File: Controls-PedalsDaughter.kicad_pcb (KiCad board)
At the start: 2 copper layers, 49.2 x 70.5 mm, 54 parts, among them J1 Brake Pos. Sensor, J2 Accel Pos. Sensor, J3 PeripheralCANConnector, J4 Conn_01x02, J5 PeripheralCANConnector, U1 RI3-1205S, U2 PeripheralSOM, U3 TLV9301xDCK, U4 TLV70130DBVR, U5 AMC1300BDWV, U6 TLV9301xDCK

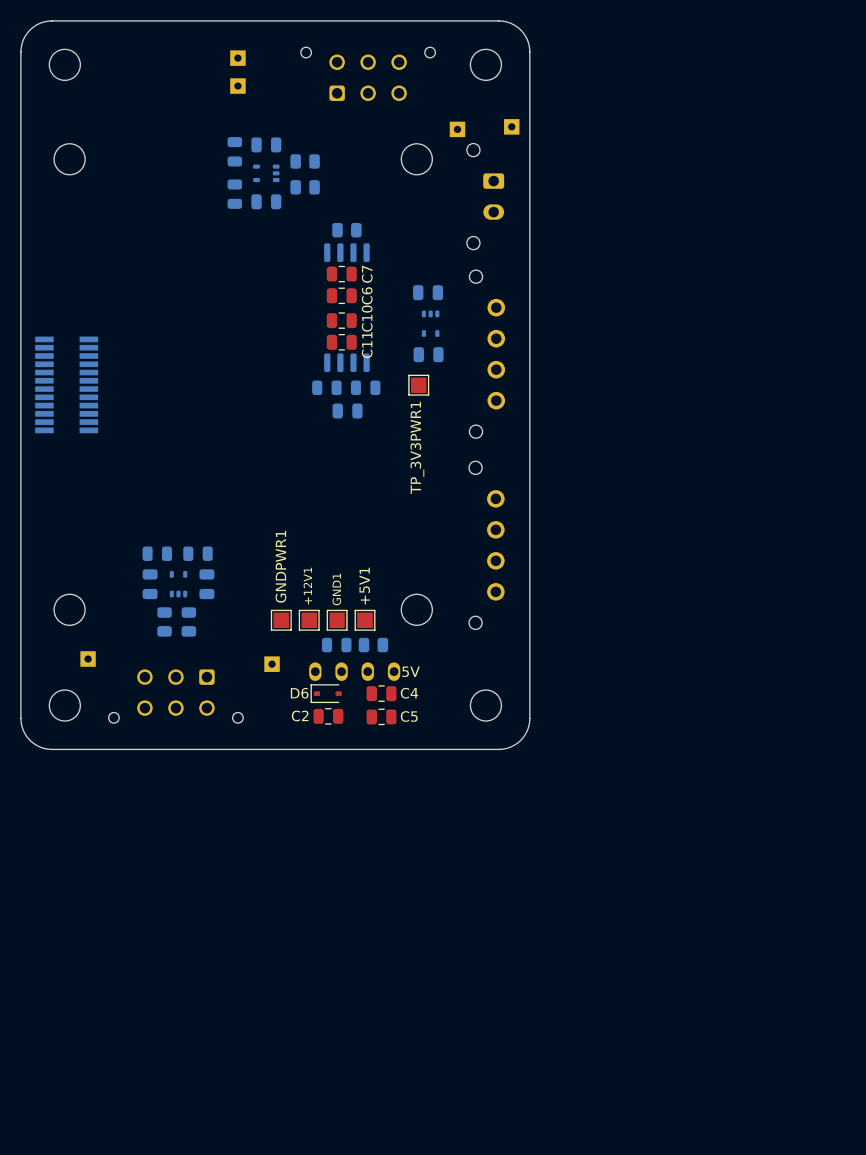
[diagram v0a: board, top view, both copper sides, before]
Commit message: thanks ravi <3
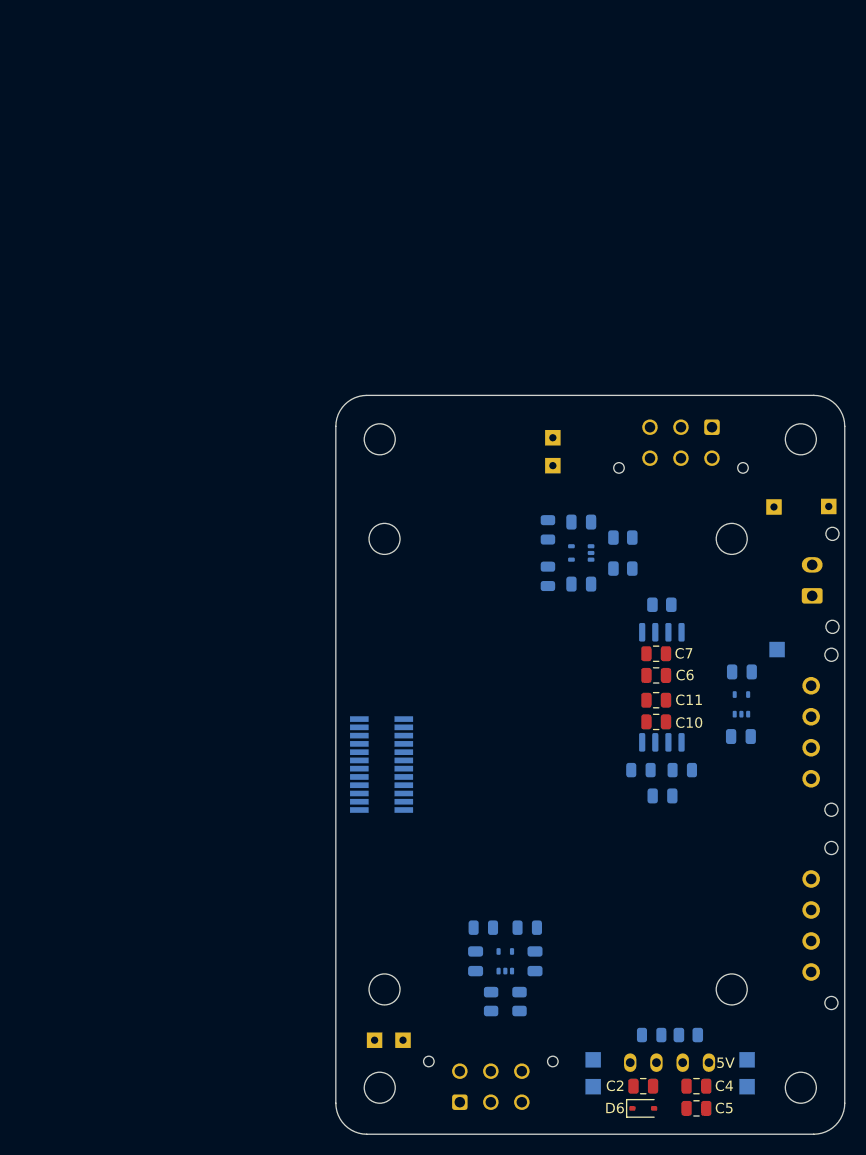
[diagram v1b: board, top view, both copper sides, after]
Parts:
- +12V1, +5V1, GND1, GNDPWR1, TP_3V3PWR1: moved to B.Cu
- moved GND1 60.1 mm to (162.3, 131.1), turned to 0 degrees
- moved +5V1 56.4 mm to (162.3, 128.5)
- moved J3 55.0 mm to (168.5, 120.0), turned to 90 degrees
- moved J5 54.8 mm to (168.5, 101.3), turned to 90 degrees
- moved GNDPWR1 54.3 mm to (147.4, 131.1), turned to 0 degrees
- moved C1 52.5 mm to (161.7, 97.2), turned to 180 degrees
- moved +12V1 50.6 mm to (147.4, 128.5), turned to 180 degrees
- moved J4 50.6 mm to (168.6, 83.6), turned to 90 degrees
- moved D6 50.4 mm to (152.2, 133.2)
- moved C10 49.3 mm to (153.5, 95.8)
- moved R4 48.7 mm to (140.2, 122.9)
- moved C4 48.7 mm to (157.4, 131.1)
- moved C5 48.6 mm to (157.4, 133.2)
- moved U1 48.6 mm to (154.8, 128.8)
- moved J1 48.6 mm to (158.9, 67.3), turned to 180 degrees
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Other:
- board size 49.2 x 70.5 mm -> 49.2 x 71.5 mm
